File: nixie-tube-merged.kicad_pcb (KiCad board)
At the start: 2 copper layers, 99.8 x 97.5 mm, 0 parts

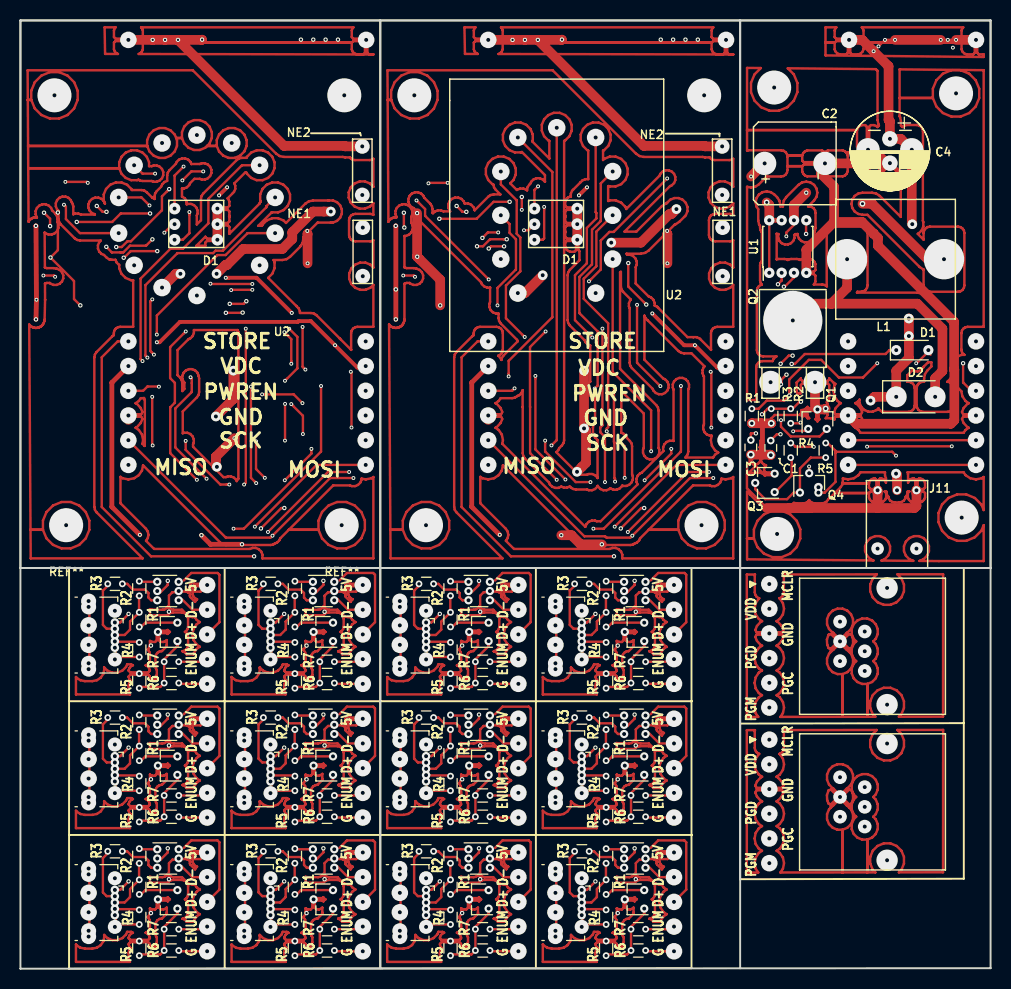
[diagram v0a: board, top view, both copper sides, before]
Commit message: finalized everything and ready to send out
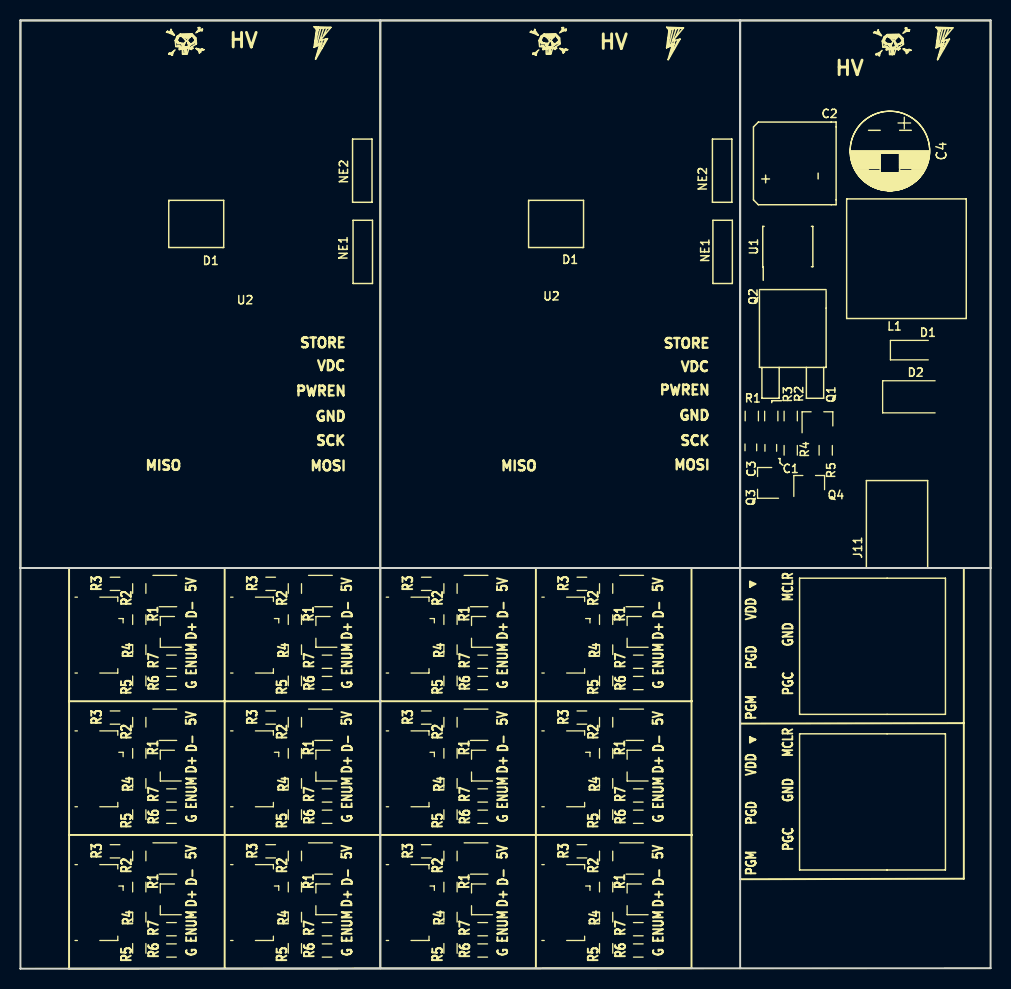
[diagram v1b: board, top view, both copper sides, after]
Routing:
- net (no net): track 5710.5 -> 0.00 mm, vias 964 -> 0
